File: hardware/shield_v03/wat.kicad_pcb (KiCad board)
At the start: 2 copper layers, 42 parts, among them J1 GS2, J2 GS2, J3 GS2, J4 Conn_02x05, J5 Conn_02x05, P1 V_IN, P2 PINZA_1, P3 PINZA_2, P4 PINZA_3, P5 PINZA_4, P6 PINZA_5, P7 PINZA_6, P8 PINZA_7, U1 LM358, U2 NANO

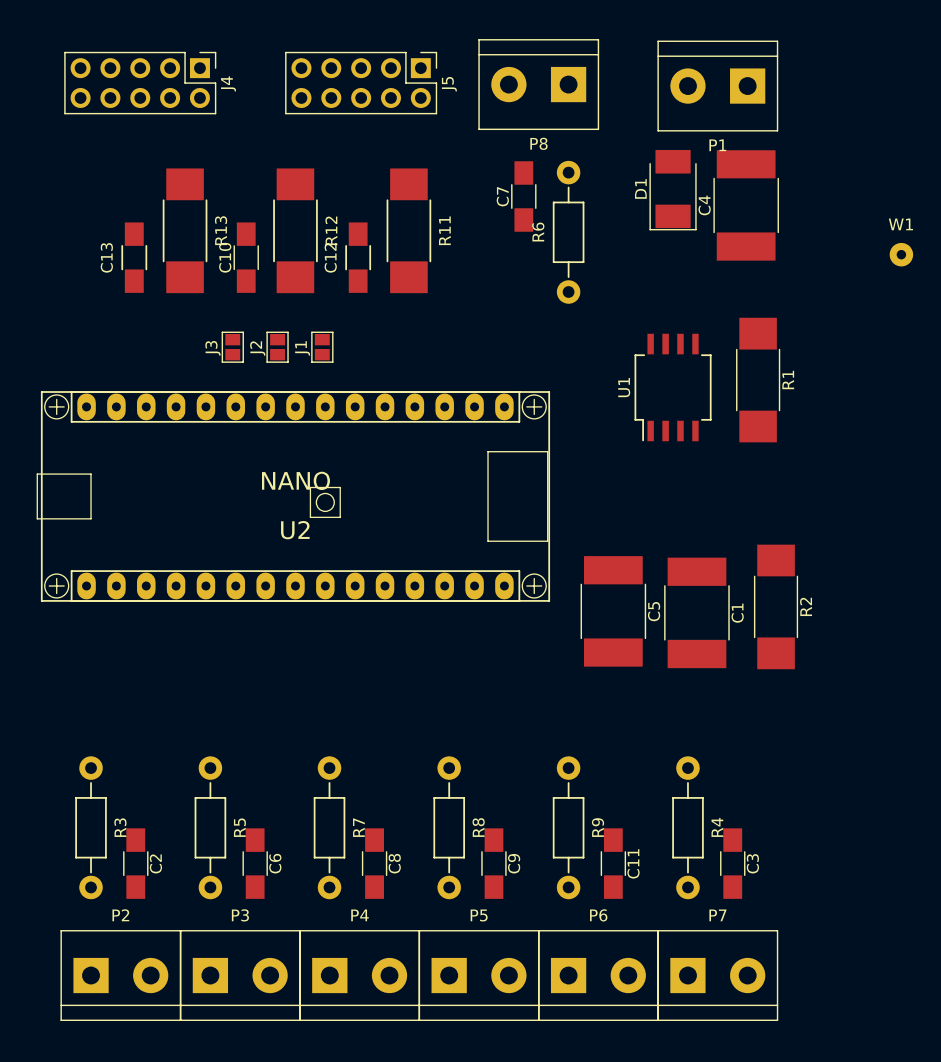
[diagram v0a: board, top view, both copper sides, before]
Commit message: desarrollo hardware
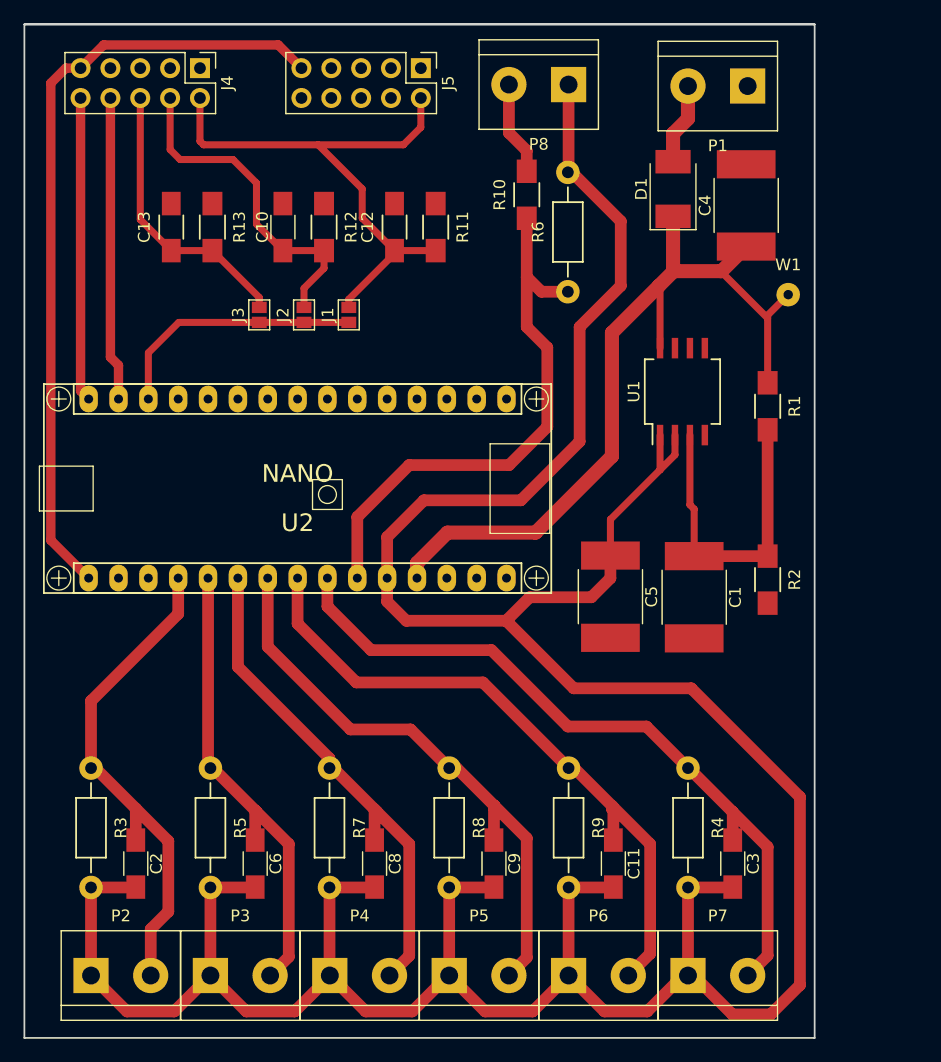
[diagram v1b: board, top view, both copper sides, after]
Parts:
- removed C7: 100nF, Capacitors_SMD:C_1206_HandSoldering
- added R10: 10k, Resistors_SMD:R_1206_HandSoldering, F.Cu at (103.5, 88.5)
- J4, J5: value Conn_02x05 -> Conn_02x05_Odd_Even
- R1, R11, R12, R13, R2: footprint Resistors_SMD:R_2512_HandSoldering -> Resistors_SMD:R_1206_HandSoldering
- R6: value 10k -> 1k
- moved W1 10.2 mm to (125.8, 97.0)
- moved C13 4.08 mm to (73.2, 91.2)
- moved C10 4.06 mm to (82.8, 91.2)
- moved C12 4.04 mm to (92.2, 91.2)
- moved J1 3.55 mm to (88.4, 98.7)
- moved J2 3.55 mm to (84.5, 98.7)
- moved J3 3.55 mm to (80.7, 98.7)
- moved R12 2.45 mm to (86.2, 91.2)
- moved R2 2.43 mm to (124.0, 121.2)
- moved R1 2.38 mm to (124.0, 106.5)
- moved R13 2.35 mm to (76.8, 91.2)
- moved R11 2.30 mm to (95.8, 91.2)
- moved C1 1.35 mm to (117.8, 122.8)
- moved C5 1.27 mm to (110.6, 122.7)
- moved U1 0.87 mm to (116.8, 105.2)
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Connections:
- P8 pad 2: /intensidad_7 -> Net-(P8-Pad2)
- R6 pad 1: /intensidad_7 -> /voltage_1
- U2 pad 25: /intensidad_7 -> /voltage_1
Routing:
- net /v_referencia: track 0.00 -> 288.3 mm
- net VCC: track 0.00 -> 70.7 mm
- net /sck: track 0.00 -> 67.2 mm
- net /intensidad_6: track 0.00 -> 62.4 mm
- net /intensidad_5: track 0.00 -> 56.8 mm
- net /intensidad_4: track 0.00 -> 50.5 mm
- net /esp_d2: track 0.00 -> 47.4 mm
- net /voltage_1: track 0.00 -> 47.0 mm
- net /intensidad_3: track 0.00 -> 43.6 mm
- net /intensidad_1: track 0.00 -> 43.1 mm
- net /intensidad_2: track 0.00 -> 40.1 mm
- net /esp_d1: track 0.00 -> 28.6 mm
- net Net-(C1-Pad1): track 0.00 -> 27.5 mm
- net /mosi: track 0.00 -> 25.9 mm
- net /miso: track 0.00 -> 25.9 mm
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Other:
- board outline added: 67.2 x 86.2 mm
